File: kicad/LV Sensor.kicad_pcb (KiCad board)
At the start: 2 copper layers, 42 parts, among them U1 AP63205WU-7, U10 LM2662MX/NOPB, U2 XMSM0C1104SPW20R, U3 FT231XS-R, U4 AP63203WU-7, U5 TLV77325PDBVR, U6 MCP2518FD-xJHA, U7 DSC1001DL5-020.0000T, U8 ADS114S06BIPBSR, U9 ATA6561-GAQW-N

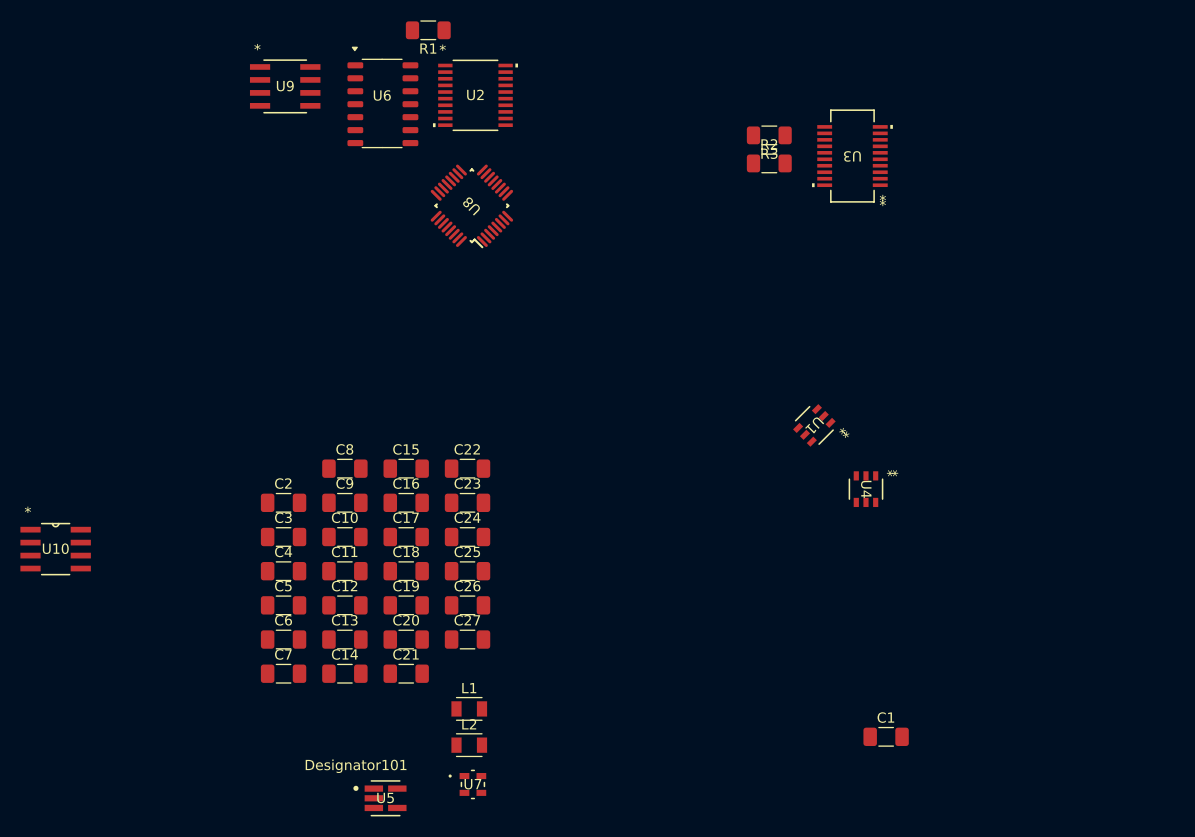
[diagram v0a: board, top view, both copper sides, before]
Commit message: 5y5y
45y45

Co-Authored-By: Manish Shrestha <manish.shr006@gmail.com>
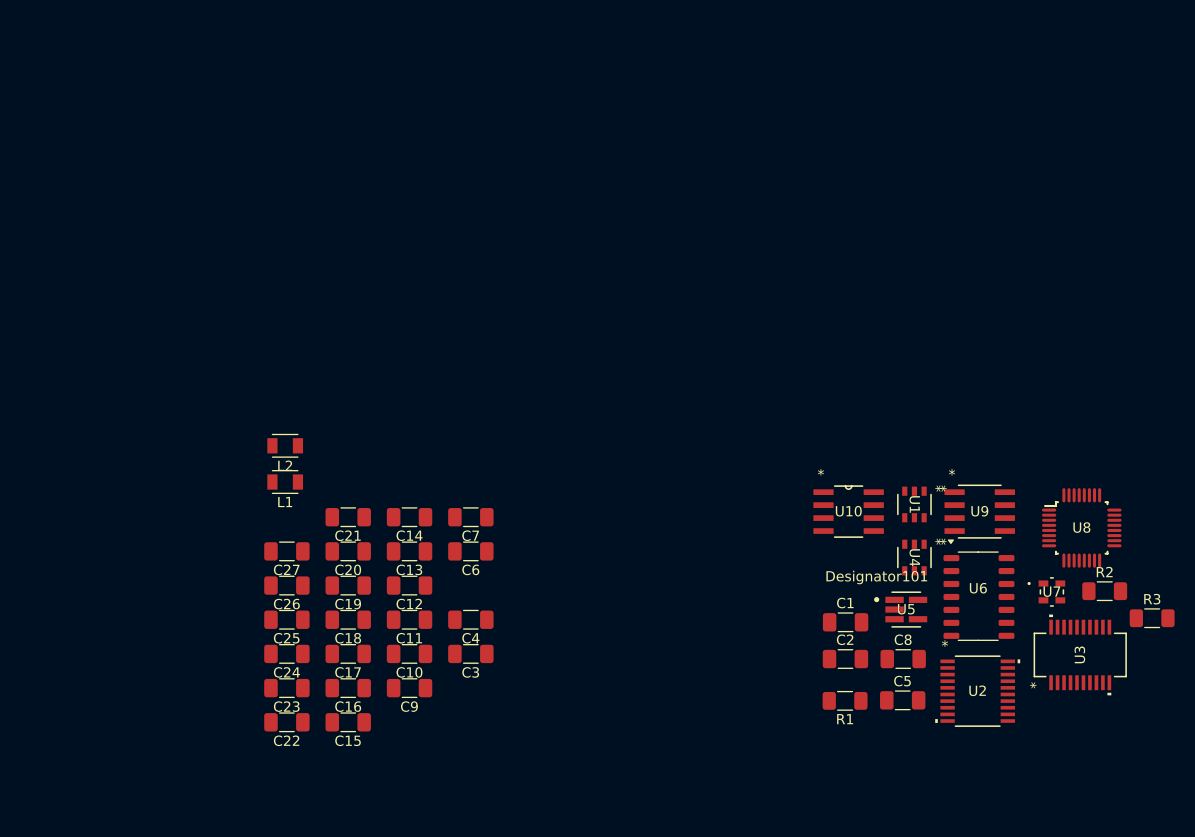
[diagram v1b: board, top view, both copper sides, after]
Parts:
- U2: value XMSM0C1104SPW20R -> MCU
- moved U9 79.8 mm to (168.0, 78.0)
- moved U10 77.8 mm to (155.2, 78.0)
- moved R1 77.4 mm to (154.8, 96.5)
- moved U2 76.4 mm to (167.8, 95.6)
- moved U6 75.8 mm to (167.8, 86.3)
- moved U8 67.6 mm to (178.0, 79.6), turned to 0 degrees
- moved C5 61.4 mm to (160.4, 96.5)
- moved R3 60.4 mm to (184.9, 88.5), turned to 0 degrees
- moved U7 59.8 mm to (175.1, 85.9)
- moved C8 57.8 mm to (160.5, 92.5)
- moved C2 57.2 mm to (154.8, 92.5)
- moved U5 54.3 mm to (160.8, 87.6)
- moved U3 53.8 mm to (177.8, 92.0), turned to 90 degrees
- moved R2 53.3 mm to (180.2, 85.8)
- moved L2 34.4 mm to (99.9, 71.5), turned to 180 degrees
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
